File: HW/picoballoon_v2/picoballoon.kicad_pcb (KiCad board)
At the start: 4 copper layers, 55 x 45 mm, 87 parts, among them IC1 MCXC141VLH, J1 EXT_DEBUGGER, J2 Conn_01x02, U1 Si4461, U2 MPL3115A2, U4 MCP9802, U5 MAX-M10S, U6 OPA333xxDBV, Y1 30M

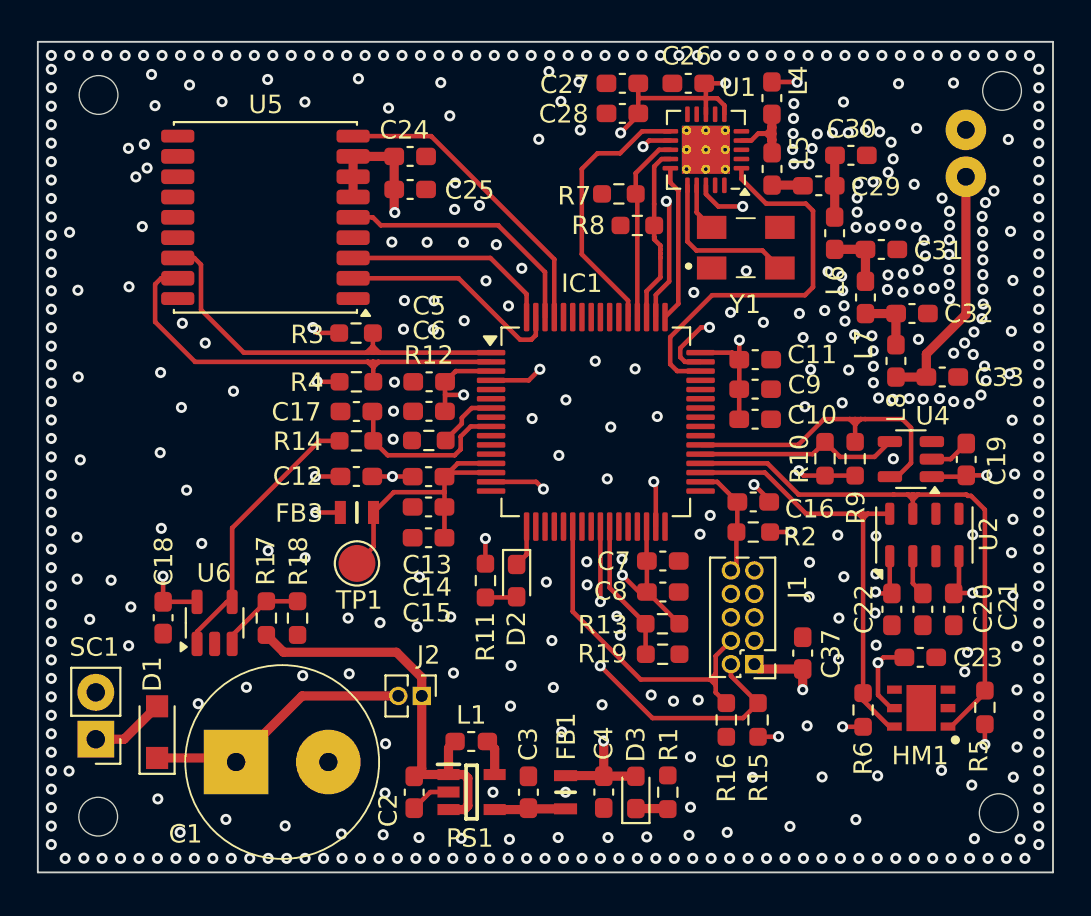
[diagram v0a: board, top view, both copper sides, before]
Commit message: PCB v2
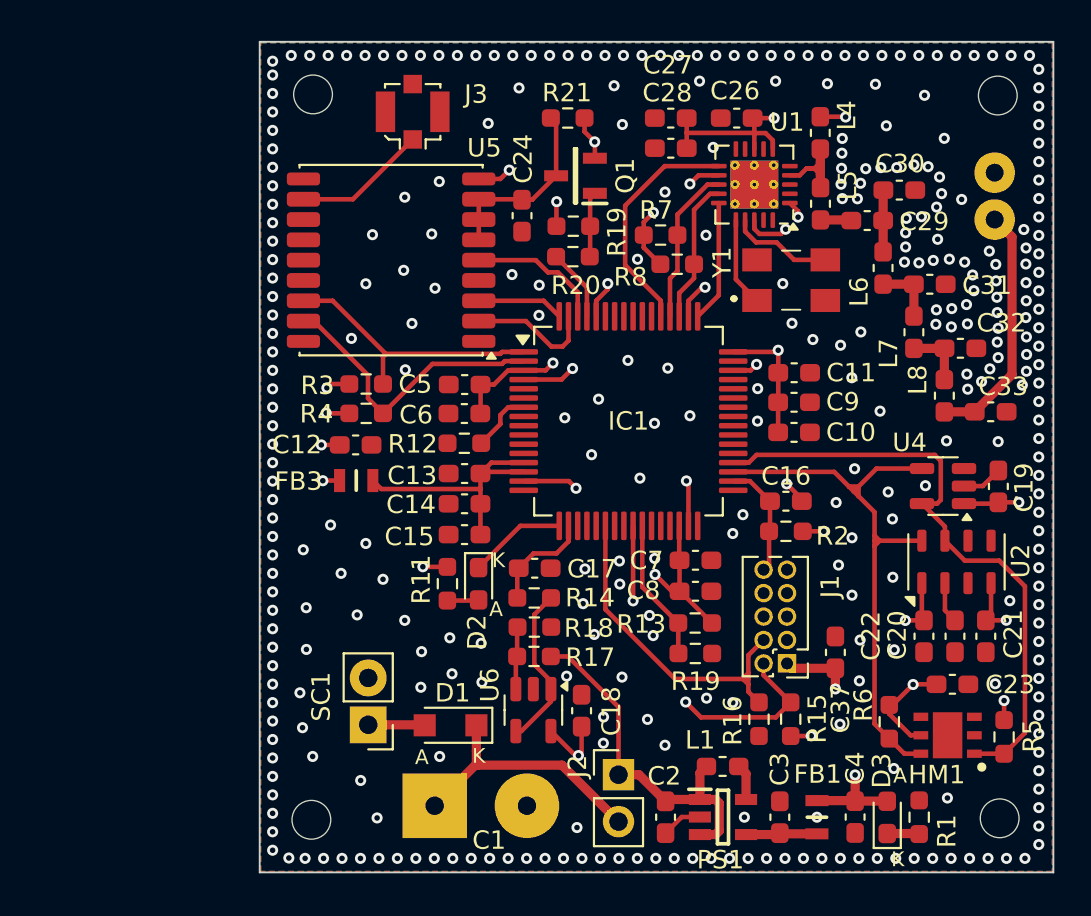
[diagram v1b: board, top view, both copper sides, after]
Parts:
- removed AE2: Antenna, Library:BNC_Connector_PCB
- removed C25: 100n, Capacitor_SMD:C_0603_1608Metric_Pad1.08x0.95mm_HandSolder
- removed R10, R9: 10k, Resistor_SMD:R_0603_1608Metric_Pad0.98x0.95mm_HandSolder
- removed TP1: +3.3VA_TP, TestPoint:TestPoint_Pad_D2.0mm
- added AE1: Antenna, Library:BNC_Connector_PCB, F.Cu at (158.6, 93.6)
- added J3: Conn_Coaxial, Connector_Coaxial:U.FL_Molex_MCRF_73412-0110_Vertical, F.Cu at (127.1, 87.8)
- added Q1: PMOS, Library:SOT95P237X112-3N, F.Cu at (135.9, 91.3)
- added R19: 10k, Resistor_SMD:R_0603_1608Metric_Pad0.98x0.95mm_HandSolder, F.Cu at (135.8, 94.0)
- added R20: 875, Resistor_SMD:R_0603_1608Metric_Pad0.98x0.95mm_HandSolder, F.Cu at (135.8, 95.7)
- added R21: 0, Resistor_SMD:R_0603_1608Metric_Pad0.98x0.95mm_HandSolder, F.Cu at (135.5, 88.1)
- C17: value xx -> 120p
- C30: value 14,35p -> 15p
- C32: value 43,06p -> 43p
- J2: footprint Connector_PinHeader_1.27mm:PinHeader_1x02_P1.27mm_Vertical -> Connector_PinHeader_2.54mm:PinHeader_1x02_P2.54mm_Vertical
- L4: value 552n -> 480n
- L6: value 106n -> 110n
- L7, L8: value 74,74n -> 75n
- R11: value 300 -> 470
- moved C18 23.2 mm to (136.2, 120.2), turned to 90 degrees
- moved U6 17.9 mm to (133.6, 120.2), turned to -90 degrees
- moved D1 15.9 mm to (129.1, 121.0), turned to 180 degrees
- moved SC1 14.8 mm to (124.7, 121.0)
- moved R17 14.6 mm to (133.7, 117.3), turned to 180 degrees
- moved C2 13.7 mm to (140.8, 126.0)
- moved C3 13.7 mm to (147.0, 126.0)
- moved C4 13.7 mm to (151.1, 126.0)
- moved D3 13.7 mm to (152.8, 126.0)
- moved L1 13.7 mm to (143.9, 123.3)
- moved R1 13.7 mm to (154.5, 126.0)
- moved PS1 13.7 mm to (143.9, 126.0)
- moved FB1 13.7 mm to (149.0, 126.0)
- moved C17 12.9 mm to (133.7, 112.5), turned to 0 degrees
- moved R14 12.9 mm to (133.7, 114.1), turned to 180 degrees
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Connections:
- C17 pad 1: Net-(IC1-PTE20) -> Net-(IC1-PTE30)
- C24 pad 1: +3.3V -> Net-(Q1-D)
- IC1 pad 18: unconnected-(IC1-PTE30-Pad18) -> Net-(IC1-PTE30)
- IC1 pad 37: /SCL_TEMP -> unconnected-(IC1-PTB2-Pad37)
- IC1 pad 38: /SDA_TEMP -> unconnected-(IC1-PTB3-Pad38)
- IC1 pad 60: unconnected-(IC1-PTD3-Pad60) -> /GNSS_RESET
- IC1 pad 61: /GNSS_RESET -> /GNSS_EN
- IC1 pad 9: Net-(IC1-PTE20) -> unconnected-(IC1-PTE20-Pad9)
- R14 pad 2: Net-(IC1-PTE20) -> Net-(IC1-PTE30)
- U4 pad 4: /SCL_TEMP -> /SCL_SENS
- U4 pad 5: /SDA_TEMP -> /SDA_SENS
- U5 pad 6: +3.3V -> Net-(Q1-D)
- U5 pad 7: +3.3V -> Net-(Q1-D)
- U5 pad 8: +3.3V -> Net-(Q1-D)
- Y1 pad 1: Net-(U1-XIN) -> Net-(U1-XOUT)
- Y1 pad 2: Net-(U1-XOUT) -> GND
- Y1 pad 4: GND -> Net-(U1-XIN)
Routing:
- net /SDA_TEMP: track 17.6 -> 0.00 mm
- net /SCL_TEMP: track 11.2 -> 0.00 mm
- net Net-(Q1-D): track 0.00 -> 10.2 mm
- net /SDN: track 21.4 -> 11.3 mm, vias 0 -> 2
- net Net-(IC1-PTE20): track 9.30 -> 0.00 mm
- net /GNSS_SCL: track 24.4 -> 15.9 mm
- net /GNSS_SDA: track 22.5 -> 14.9 mm
- net /SCL_SENS: track 24.3 -> 31.8 mm
- net Net-(J3-In): track 0.00 -> 7.26 mm
- net /GNSS_RX: track 11.4 -> 4.71 mm
- net /GNSS_EXTINT: track 14.1 -> 7.39 mm
- net GND: track 22.8 -> 16.5 mm, vias 447 -> 336
- net /ADC: track 15.0 -> 8.92 mm
- net Net-(IC1-PTE30): track 0.00 -> 5.78 mm
- net /GNSS_TX: track 12.4 -> 6.88 mm
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- added copper zone on In2.Cu, net +3.3V
- added copper zone on B.Cu, net GND
- added copper zone on F.Cu, net GND
- added copper zone on In1.Cu, net GND
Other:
- board size 55 x 45 mm -> 43 x 45 mm
- board text added: "A"
- board text added: "GND"
- board text added: "K"
- board text added: "Vojtech Piroch Picoballoon v2 vojta.piroch@gmail.com 2024/25"
- board text removed: "Vojtech Piroch Picoballoon v1 2024/25"
